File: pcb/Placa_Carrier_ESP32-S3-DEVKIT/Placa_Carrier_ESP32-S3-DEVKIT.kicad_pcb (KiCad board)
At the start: 2 copper layers, 152.3 x 50.6 mm, 45 parts, among them J1 12V IN, J2 AN_IN, J3 RELE, J4 CAN, J5 DevKit_J1, J6 DevKit_J3, J7 EXP_J1, J8 EXP_J3, K1 SRD-05VDC, Q1 BC817, SW1 SW_Push, SW2 SW_Push, U1 AMS1117-ADJ, U3 MCP2562-E-SN

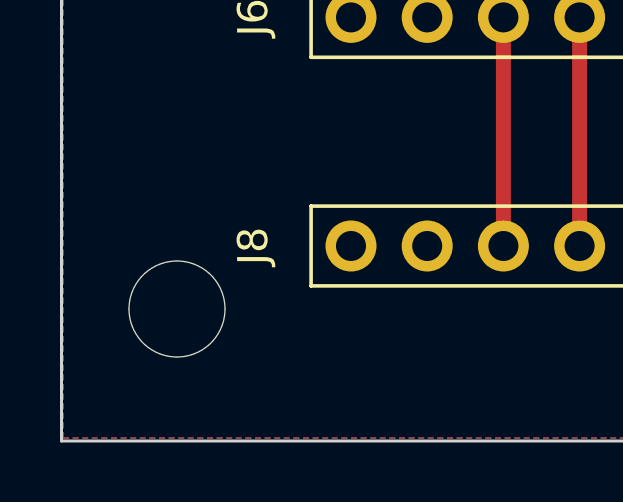
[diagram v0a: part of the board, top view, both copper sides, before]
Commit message: Sube PCB ruteado sin refinar
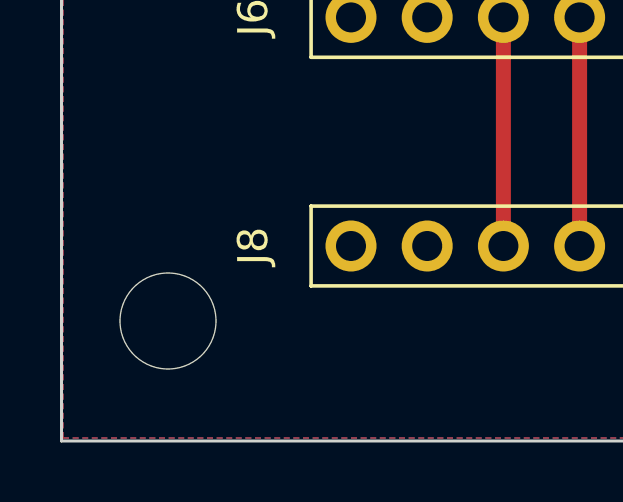
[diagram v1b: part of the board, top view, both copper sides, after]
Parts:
- moved H2 0.50 mm to (103.4, 104.2)
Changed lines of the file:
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@@
 	(footprint "MountingHole:MountingHole_3.2mm_M3"
 		(layer "F.Cu")
-		(at 103.7 103.8)
+		(at 103.4 104.2)
 		(descr "Mounting Hole 3.2mm, no annular, M3")
 		(tags "mounting hole 3.2mm no annular m3")
